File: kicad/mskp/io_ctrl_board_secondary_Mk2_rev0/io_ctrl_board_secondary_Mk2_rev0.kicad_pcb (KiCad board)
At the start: 2 copper layers, 29 parts, among them J1 USB_C_I2C_input, J2 Keypad_matrix_connector_JST, J3 OLED_128x64, J4 I2C_aux_JST, J5 RJ45_SPI_I2C_input, J6 SPI_aux_JST, J7 I2C_aux_pads, U1 MCP23017_SP, U2 AMS1117-3v3

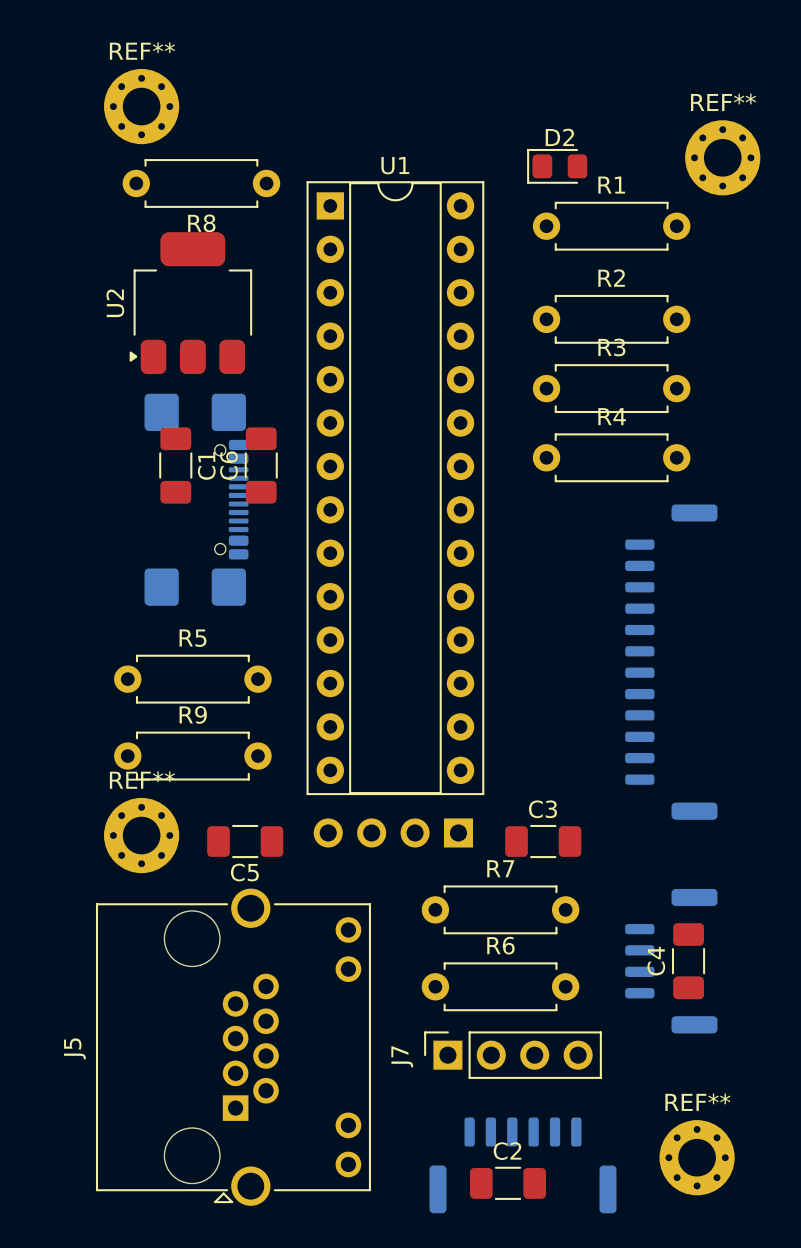
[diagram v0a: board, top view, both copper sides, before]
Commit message: Continues work with rough PCB outlines
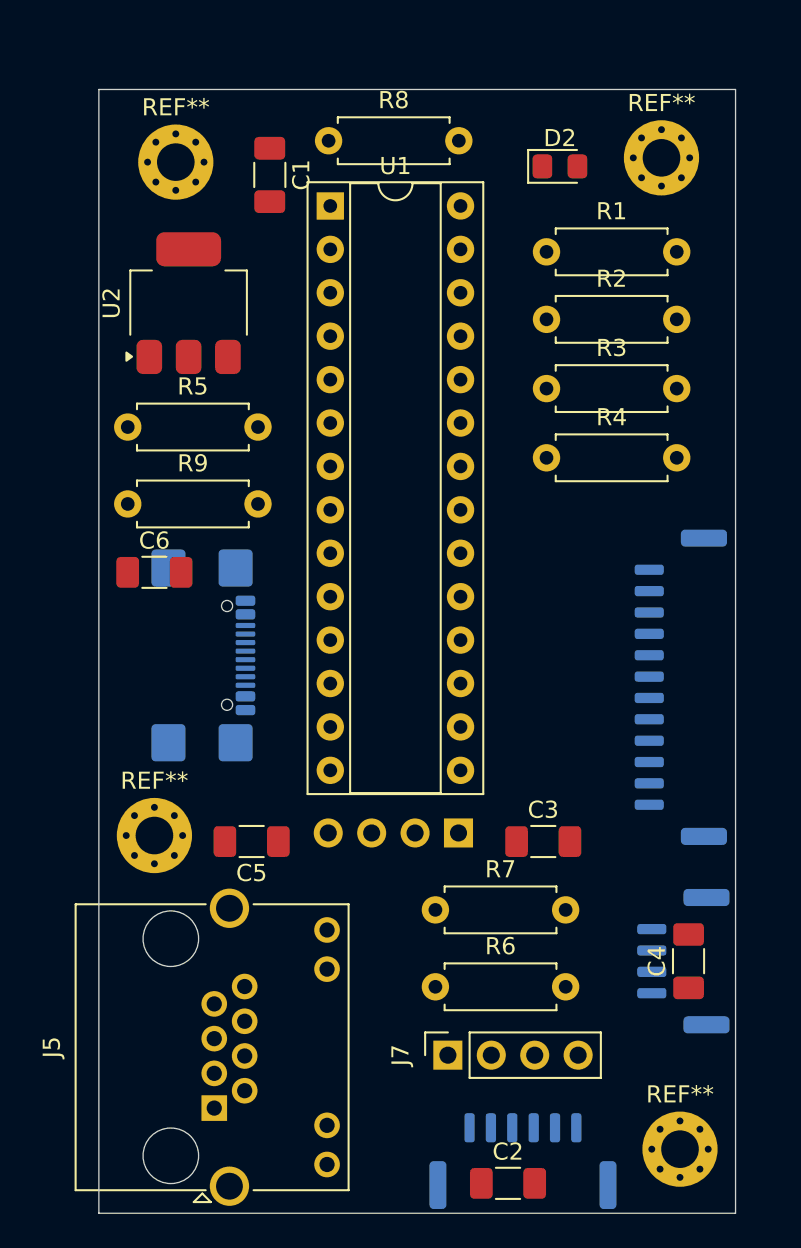
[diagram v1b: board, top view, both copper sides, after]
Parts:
- moved C1 17.9 mm to (123.0, 61.5)
- moved R5 14.8 mm to (114.7, 76.2)
- moved R9 14.8 mm to (114.7, 80.8)
- moved J1 9.12 mm to (117.9, 89.6)
- moved C6 8.84 mm to (116.2, 84.8), turned to 0 degrees
- moved R8 4.41 mm to (126.4, 59.5), turned to 0 degrees
- moved REF** 3.82 mm to (117.5, 60.8)
- moved REF** 3.58 mm to (145.9, 60.5)
- moved J2 1.57 mm to (147.1, 91.5)
- moved R1 1.50 mm to (139.2, 66.0)
- moved J5 1.25 mm to (119.8, 116.1)
- moved REF** 1.12 mm to (147.0, 118.5)
- moved REF** 0.75 mm to (116.2, 100.2)
- moved J4 0.70 mm to (147.2, 107.5)
- moved C5 0.38 mm to (121.9, 100.5)
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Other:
- board outline added: 37.2 x 65.8 mm
